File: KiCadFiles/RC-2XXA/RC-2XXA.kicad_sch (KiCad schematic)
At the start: 259 parts, among them J1 Conn_01x01_Pin, J2 Conn_01x04_Pin, J3 Conn_01x04_Pin, J4 Conn_01x07_Socket, J5 Conn_01x07_Socket, SW1 SW_DPST_x2, SW2 SW_DPST_x2, U1 TLV74318PDBVR, U2 PMW3360DM-T2QU, U3 TPD4E05U06DQAR, U4 STM32F072CBTx, U5 XC6206PxxxMR

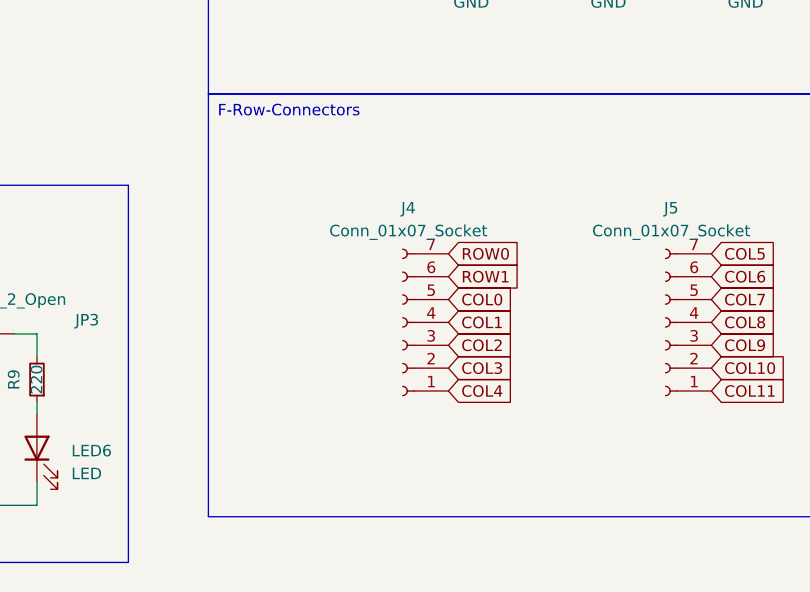
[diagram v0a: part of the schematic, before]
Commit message: Refactor code structure for improved readability and maintainability
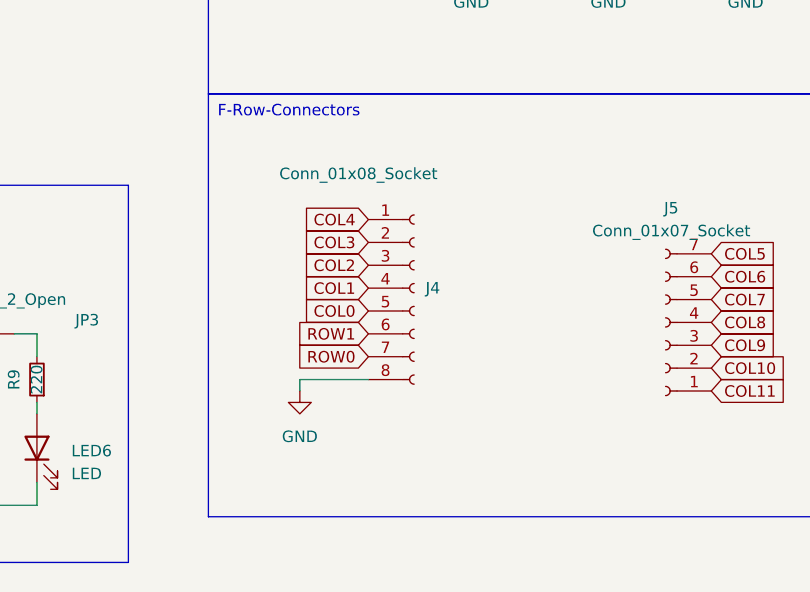
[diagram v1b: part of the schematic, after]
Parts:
- removed J4: Conn_01x07_Socket, Connector_JST:JST_SH_SM07B-SRSS-TB_1x07-1MP_P1.00mm_Horizontal, symbol Connector:Conn_01x07_Socket
- added J4: Conn_01x08_Socket, Connector_JST:JST_SH_SM08B-SRSS-TB_1x08-1MP_P1.00mm_Horizontal, symbol Connector:Conn_01x08_Socket
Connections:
- net COL0: now also J4.5 (Pin_5)
- net COL1: now also J4.4 (Pin_4)
- net COL2: now also J4.3 (Pin_3)
- net COL3: now also J4.2 (Pin_2)
- net COL4: now also J4.1 (Pin_1)
- net GND: now also J4.8 (Pin_8)
- net ROW0: now also J4.7 (Pin_7)
- net ROW1: now also J4.6 (Pin_6)
